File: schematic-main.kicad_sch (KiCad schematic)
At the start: 12 parts, among them J1 Fell_Cell_IN, J2 CAN, J3 P_Valve, J4 FC Cooling, J5 Valve, J7 Axilary_Out, J9 Analog_In, P1 USB_C_Plug_USB2.0

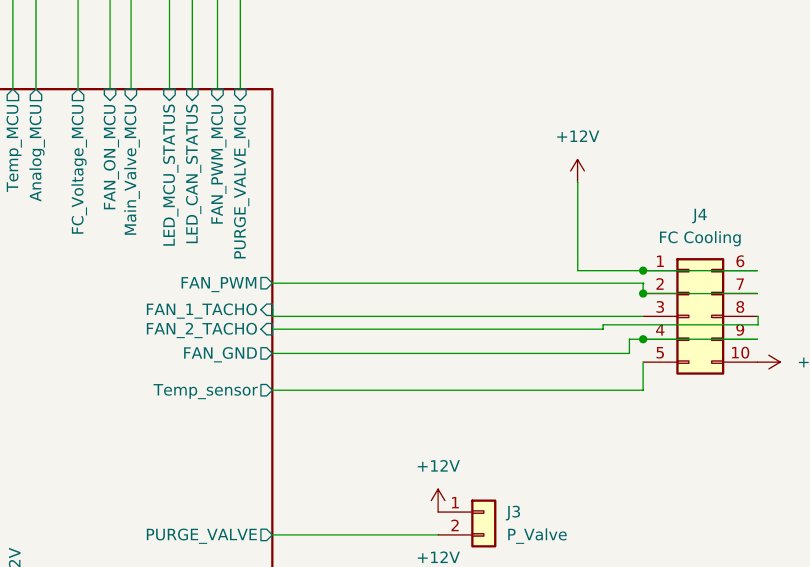
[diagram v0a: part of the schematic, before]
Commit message: porawa library
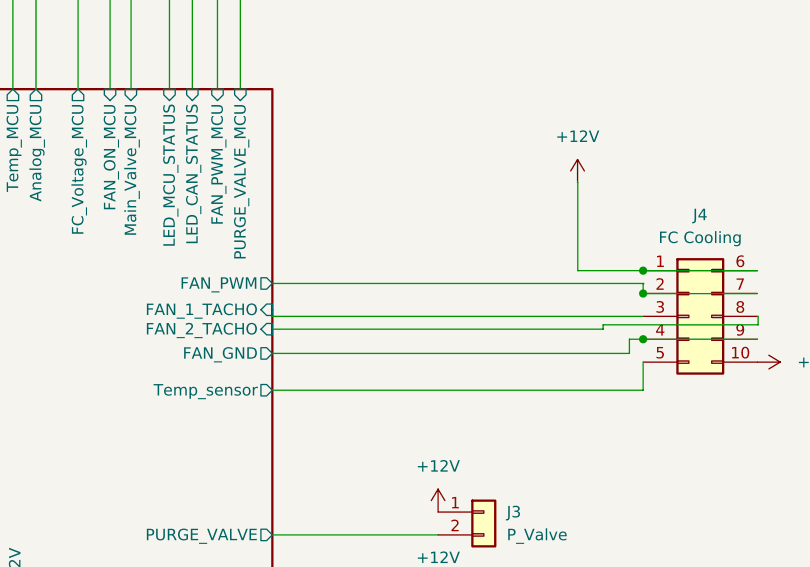
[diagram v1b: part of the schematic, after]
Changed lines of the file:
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@@
     (stroke (width 0) (type default))
   )
-  (wire (pts (xy 227.3046 125.7508) (xy 227.3046 125.7))
+  (wire (pts (xy 227.3046 125.7508) (xy 227.3046 125.73))
     (stroke (width 0) (type default))
   )
@@
     (stroke (width 0) (type default))
   )
-  (wire (pts (xy 227.3046 125.7) (xy 186.055 125.7))
+  (wire (pts (xy 227.3046 125.73) (xy 186.055 125.73))
     (stroke (width 0) (type default))
   )
@@
       (effects (font (size 1.27 1.27)) (justify left))
     )
-    (pin "FAN_PWM" output (at 186.055 125.7 0)
+    (pin "FAN_PWM" output (at 186.055 125.73 0)
       (effects (font (size 1.27 1.27)) (justify right))
     )
